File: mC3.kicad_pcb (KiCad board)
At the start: 2 copper layers, 19.7 x 31.4 mm, 36 parts, among them J1 Sh 1.0, J2 USB_C_Receptacle_PowerOnly_6P, Q1 AO3401A, SW1 SW_Push, SW2 SW_SPDT, U1 MPU-6050, U2 IP5306, U3 ESP32C3_SuperMini

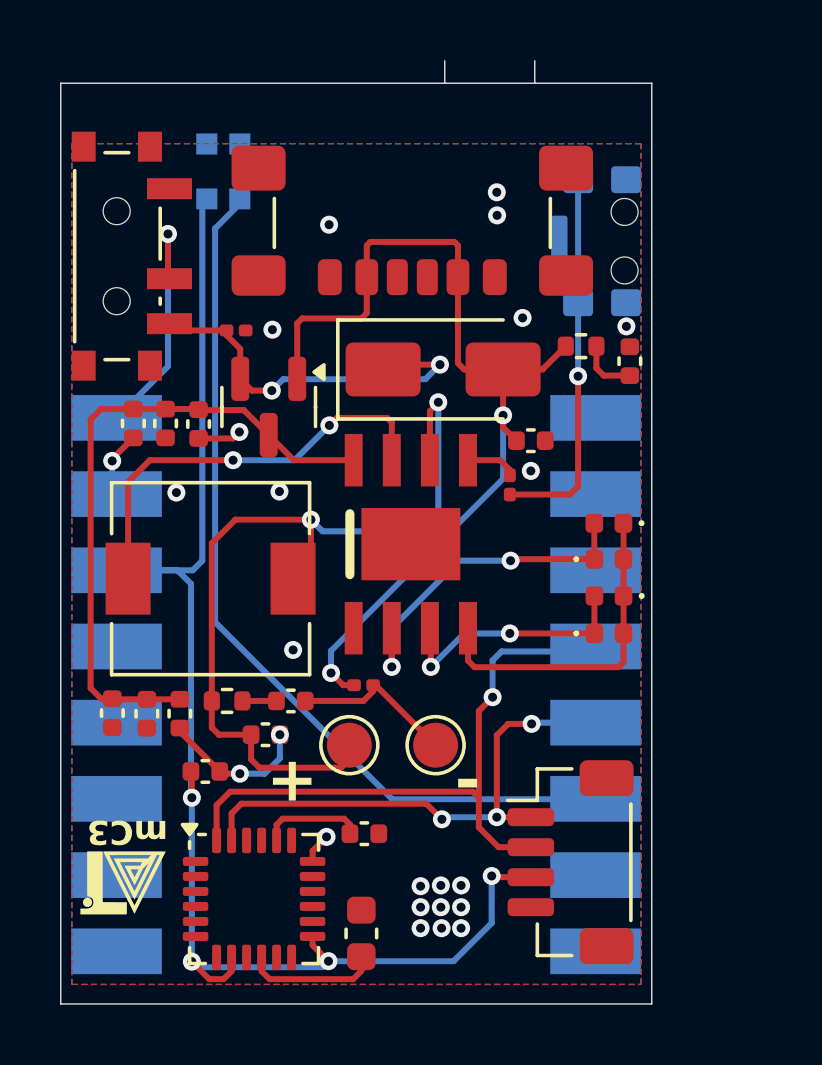
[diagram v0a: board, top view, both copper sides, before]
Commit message: Update mC3.kicad_pcb
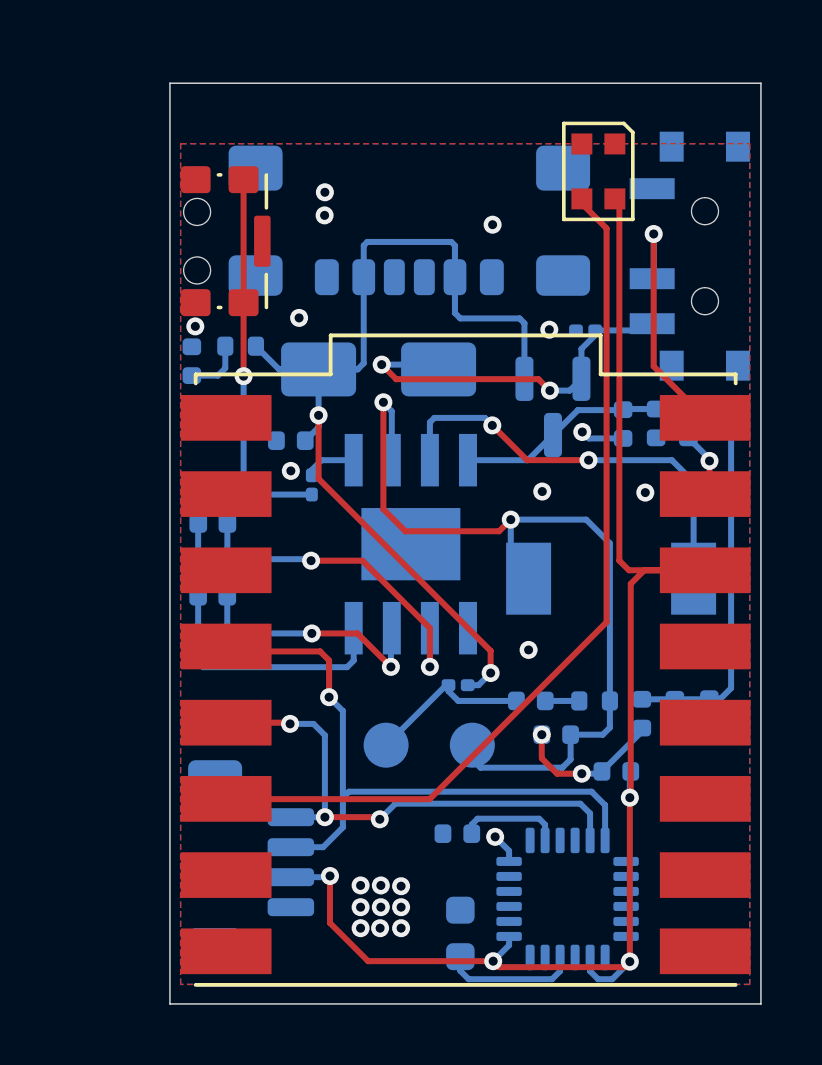
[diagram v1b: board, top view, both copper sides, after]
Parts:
- C1, C10, C11, C12, C13, C14, C2, C3, C4, C5, C6, C7, C8, C9, D2, D3, D4, D5, D6, G***, J1, J2, L1, Q1, R2, R3, R4, R5, SW2, TP1, TP2, U1, U2: moved to B.Cu
- D7, SW1, U3: moved to F.Cu
- moved C9 19.9 mm to (115.5, 40.9)
- moved G*** 19.0 mm to (115.1, 46.6), turned to 0 degrees
- moved SW2 19.0 mm to (115.0, 25.7)
- moved C8 18.5 mm to (114.8, 31.3)
- moved C10 17.6 mm to (114.4, 40.9)
- moved C12 16.3 mm to (113.7, 31.3)
- moved C13 15.4 mm to (113.3, 40.9)
- moved C2 14.6 mm to (98.3, 29.2)
- moved C11 14.2 mm to (112.6, 31.3)
- moved C14 13.7 mm to (112.4, 42.9), turned to 180 degrees
- moved L1 13.3 mm to (112.2, 36.4), turned to 180 degrees
- moved D4 13.2 mm to (99.0, 35.8), turned to 180 degrees
- moved D5 13.2 mm to (99.0, 37.0), turned to 0 degrees
- moved D6 13.2 mm to (99.0, 38.3), turned to 180 degrees
- moved D3 13.2 mm to (99.0, 34.6), turned to 0 degrees
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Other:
- board size 19.7 x 31.4 mm -> 19.7 x 30.7 mm
